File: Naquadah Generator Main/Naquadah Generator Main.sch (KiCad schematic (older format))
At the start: 15 parts, among them SW1 RESET, U1 ATmega32U4-AU, Y1 16MHz

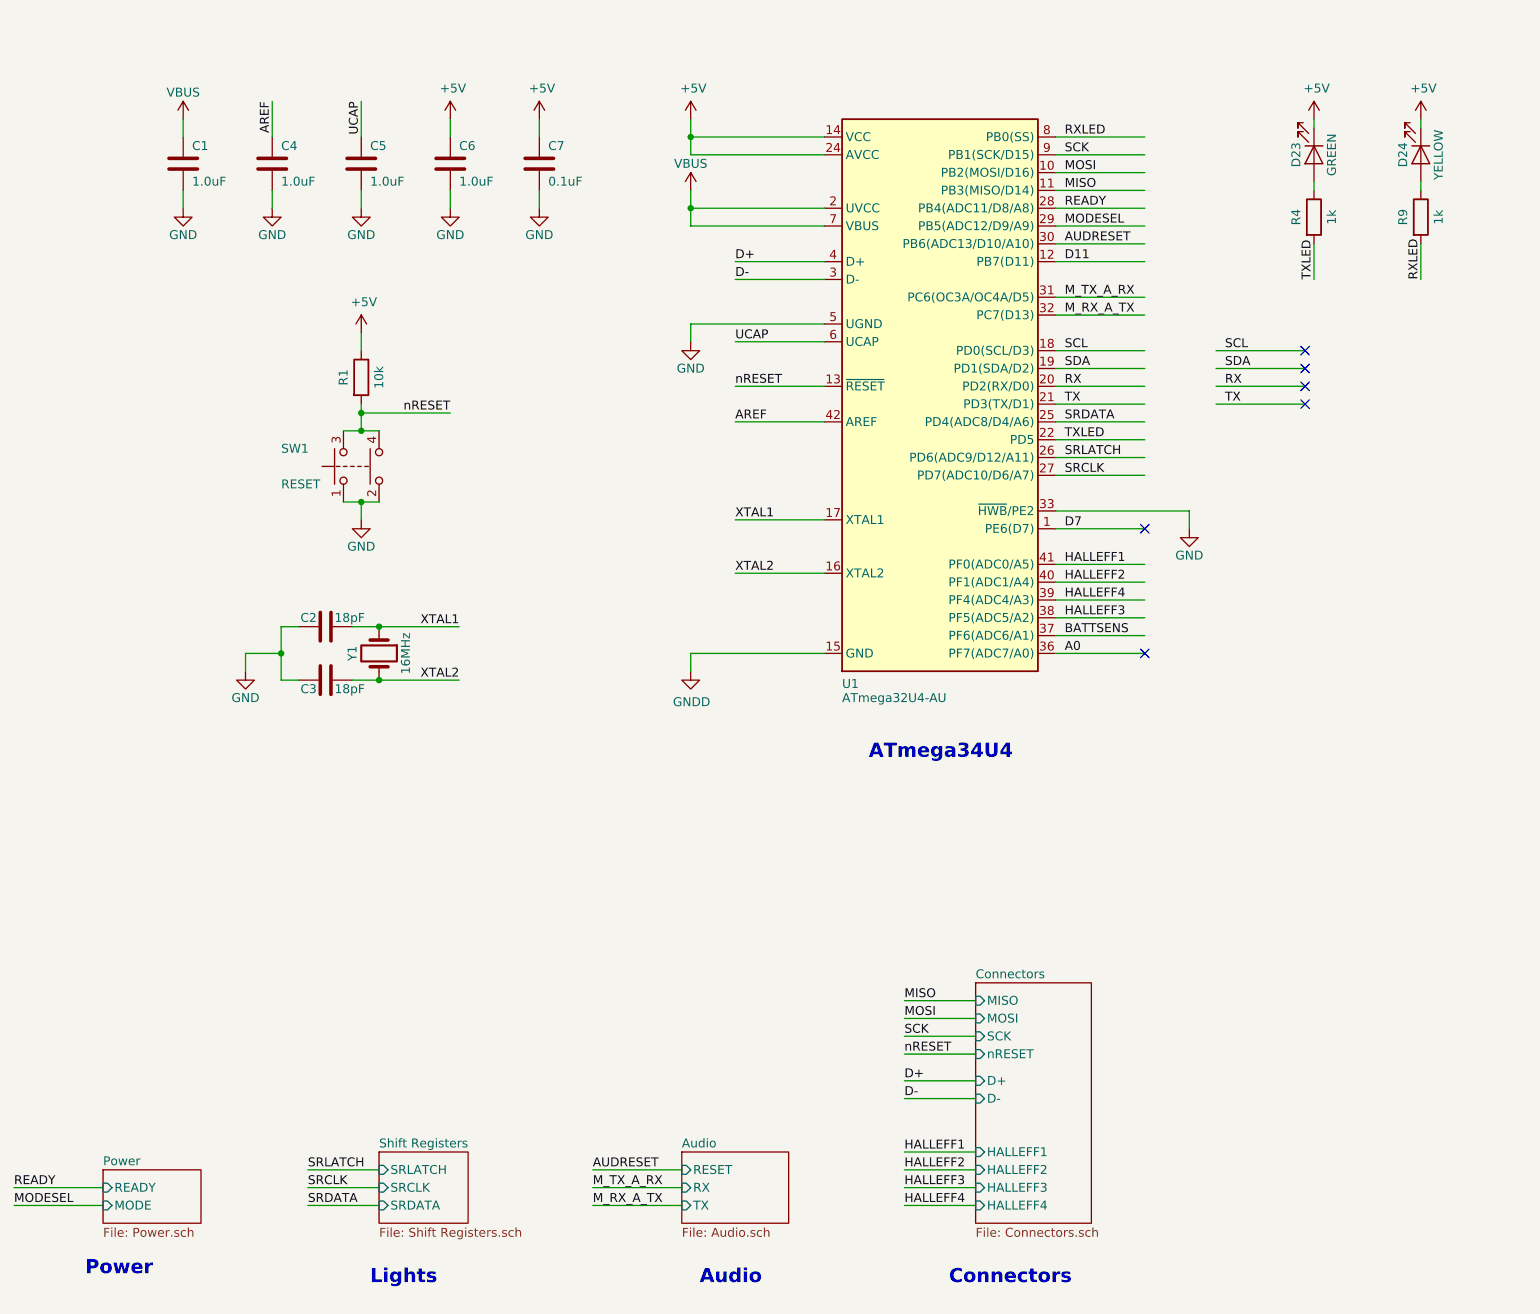
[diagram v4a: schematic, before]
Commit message: Separated digital and analog ground.
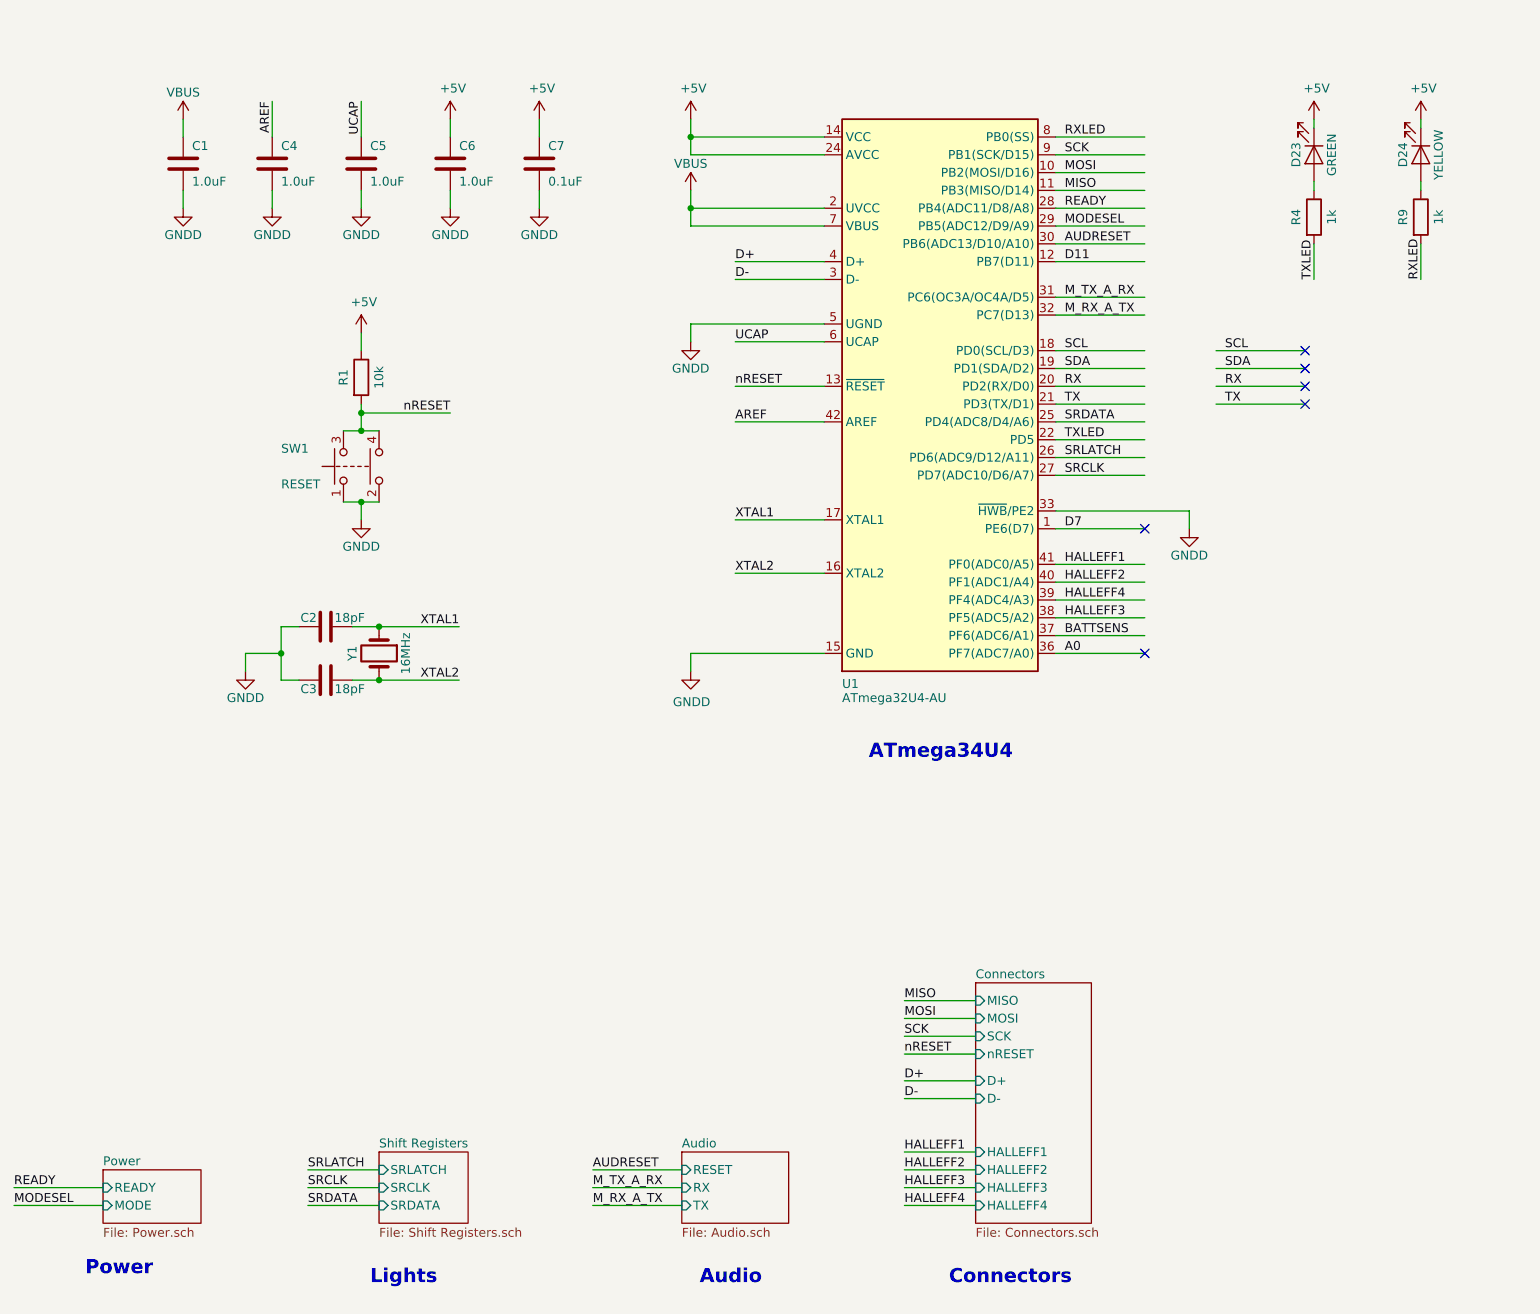
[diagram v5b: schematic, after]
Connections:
- net labels removed: GND
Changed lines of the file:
@@
 	4500 2150 4500 2250
 $Comp
-L Frequently_Used_LE:GND #PWR016
+L Frequently_Used_LE:GNDD #PWR016
 U 1 1 5EDBAB65
 P 4500 2250
 F 0 "#PWR016" H 4500 2000 50  0001 C CNN
-F 1 "GND" H 4500 2100 50  0000 C CNN
+F 1 "GNDD" H 4500 2100 50  0000 C CNN
 F 2 "" H 4500 2250 50  0001 C CNN
 F 3 "" H 4500 2250 50  0001 C CNN
@@
 $EndComp
 $Comp
-L Frequently_Used_LE:GND #PWR011
+L Frequently_Used_LE:GNDD #PWR011
 U 1 1 5EE3FE38
 P 3650 1500
 F 0 "#PWR011" H 3650 1250 50  0001 C CNN
-F 1 "GND" H 3650 1350 50  0000 C CNN
+F 1 "GNDD" H 3650 1350 50  0000 C CNN
 F 2 "" H 3650 1500 50  0001 C CNN
 F 3 "" H 3650 1500 50  0001 C CNN
@@
 $EndComp
 $Comp
-L Frequently_Used_LE:GND #PWR09
+L Frequently_Used_LE:GNDD #PWR09
 U 1 1 5EE4608D
 P 3150 1500
 F 0 "#PWR09" H 3150 1250 50  0001 C CNN
-F 1 "GND" H 3150 1350 50  0000 C CNN
+F 1 "GNDD" H 3150 1350 50  0000 C CNN
 F 2 "" H 3150 1500 50  0001 C CNN
 F 3 "" H 3150 1500 50  0001 C CNN
@@
 	3150 1000 3150 1100
 $Comp
-L Frequently_Used_LE:GND #PWR07
+L Frequently_Used_LE:GNDD #PWR07
 U 1 1 5EE499D3
 P 2650 1500
 F 0 "#PWR07" H 2650 1250 50  0001 C CNN
-F 1 "GND" H 2650 1350 50  0000 C CNN
+F 1 "GNDD" H 2650 1350 50  0000 C CNN
 F 2 "" H 2650 1500 50  0001 C CNN
 F 3 "" H 2650 1500 50  0001 C CNN
@@
 	2650 900  2650 1100
 $Comp
-L Frequently_Used_LE:GND #PWR03
+L Frequently_Used_LE:GNDD #PWR03
 U 1 1 5EE4D88E
 P 1650 1500
 F 0 "#PWR03" H 1650 1250 50  0001 C CNN
-F 1 "GND" H 1650 1350 50  0000 C CNN
+F 1 "GNDD" H 1650 1350 50  0000 C CNN
 F 2 "" H 1650 1500 50  0001 C CNN
 F 3 "" H 1650 1500 50  0001 C CNN
@@
 UCAP
 $Comp
-L Frequently_Used_LE:GND #PWR06
+L Frequently_Used_LE:GNDD #PWR06
 U 1 1 5EE53061
 P 2150 1500
 F 0 "#PWR06" H 2150 1250 50  0001 C CNN
-F 1 "GND" H 2150 1350 50  0000 C CNN
+F 1 "GNDD" H 2150 1350 50  0000 C CNN
 F 2 "" H 2150 1500 50  0001 C CNN
 F 3 "" H 2150 1500 50  0001 C CNN
@@
 Connection ~ 2650 2650
 $Comp
-L Frequently_Used_LE:GND #PWR05
+L Frequently_Used_LE:GNDD #PWR05
 U 1 1 5EE8456D
 P 2650 3250
 F 0 "#PWR05" H 2650 3000 50  0001 C CNN
-F 1 "GND" H 2650 3100 50  0000 C CNN
+F 1 "GNDD" H 2650 3100 50  0000 C CNN
 F 2 "" H 2650 3250 50  0001 C CNN
 F 3 "" H 2650 3250 50  0001 C CNN
@@
 	2200 4000 2200 3850
 $Comp
-L Frequently_Used_LE:GND #PWR01
+L Frequently_Used_LE:GNDD #PWR01
 U 1 1 5ECBCDF9
 P 2000 4100
 F 0 "#PWR01" H 2000 3850 50  0001 C CNN
-F 1 "GND" H 2000 3950 50  0000 C CNN
+F 1 "GNDD" H 2000 3950 50  0000 C CNN
 F 2 "" H 2000 4100 50  0001 C CNN
 F 3 "" H 2000 4100 50  0001 C CNN
@@
 	7300 3200 6550 3200
 $Comp
-L Frequently_Used_LE:GND #PWR0105
+L Frequently_Used_LE:GNDD #PWR0105
 U 1 1 5EE11E5E
 P 7300 3300
 F 0 "#PWR0105" H 7300 3050 50  0001 C CNN
-F 1 "GND" H 7300 3150 50  0000 C CNN
+F 1 "GNDD" H 7300 3150 50  0000 C CNN
 F 2 "" H 7300 3300 50  0001 C CNN
 F 3 "" H 7300 3300 50  0001 C CNN
